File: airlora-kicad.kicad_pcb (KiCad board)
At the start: 4 copper layers, 77 x 77 mm, 125 parts, among them IC1 BALFHB-WL-02D3, J1 12V, J10 I2C, J11 UART2, J2 Conn_Coaxial, J3 Led, J4 SHT, J5 I2C, J6 A_NO2, J7 UART1, J8 A_CO, J9 I2C, Q10 S8050, Q2 S8050, Q3 S8050, Q4 S8050, Q5 S8050, Q6 S8050, Q7 S8050, Q8 S8050, Q9 S8050, SW1 SW_Push, SW2 SW_Slide_DPDT, SW3 SW_Push, U1 TPS7A2633DRVR, U2 TPS54202DDC, U3 TPS7A2633DRVR, U4 BGS12WN6E6327, U6 STM32F103C8Tx, U7 STM32WLE5CCUx, X1 32MHZ, Y1 32.768kHz, Y2 8Mhz

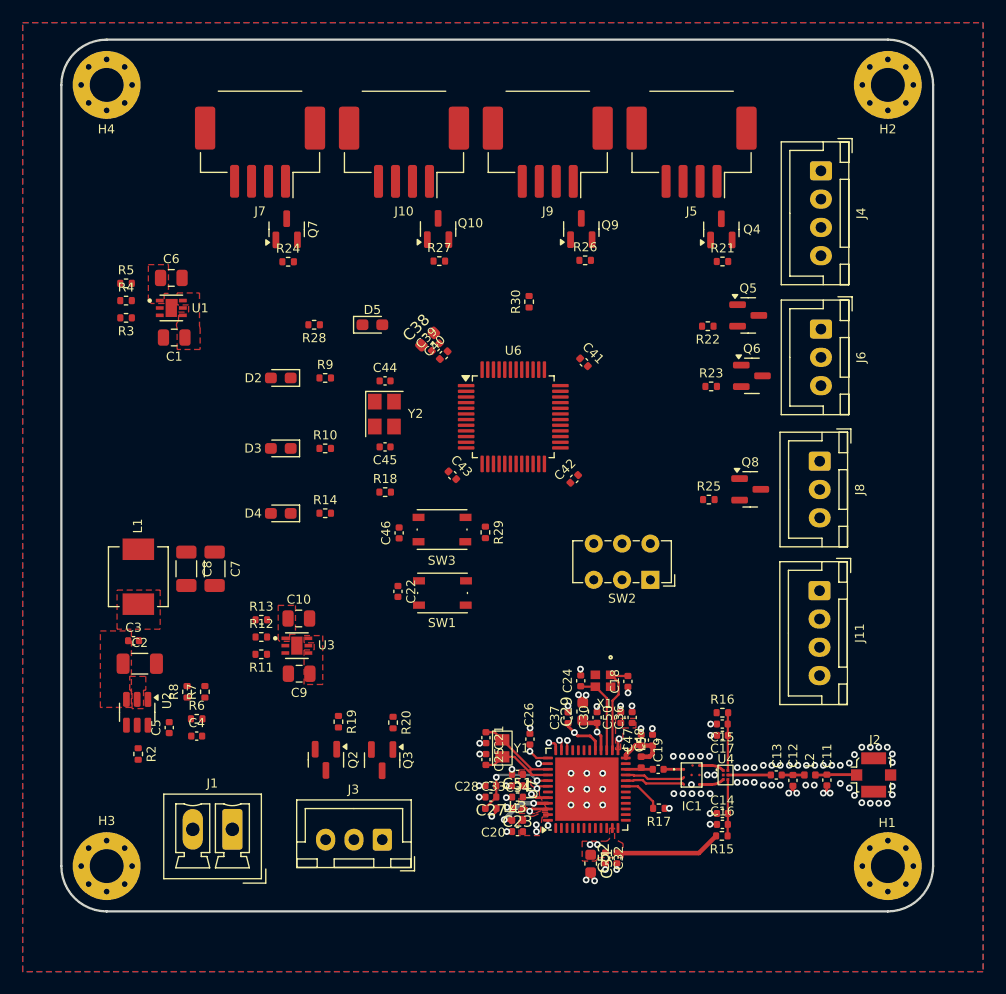
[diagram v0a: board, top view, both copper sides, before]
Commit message: Update PCB layout
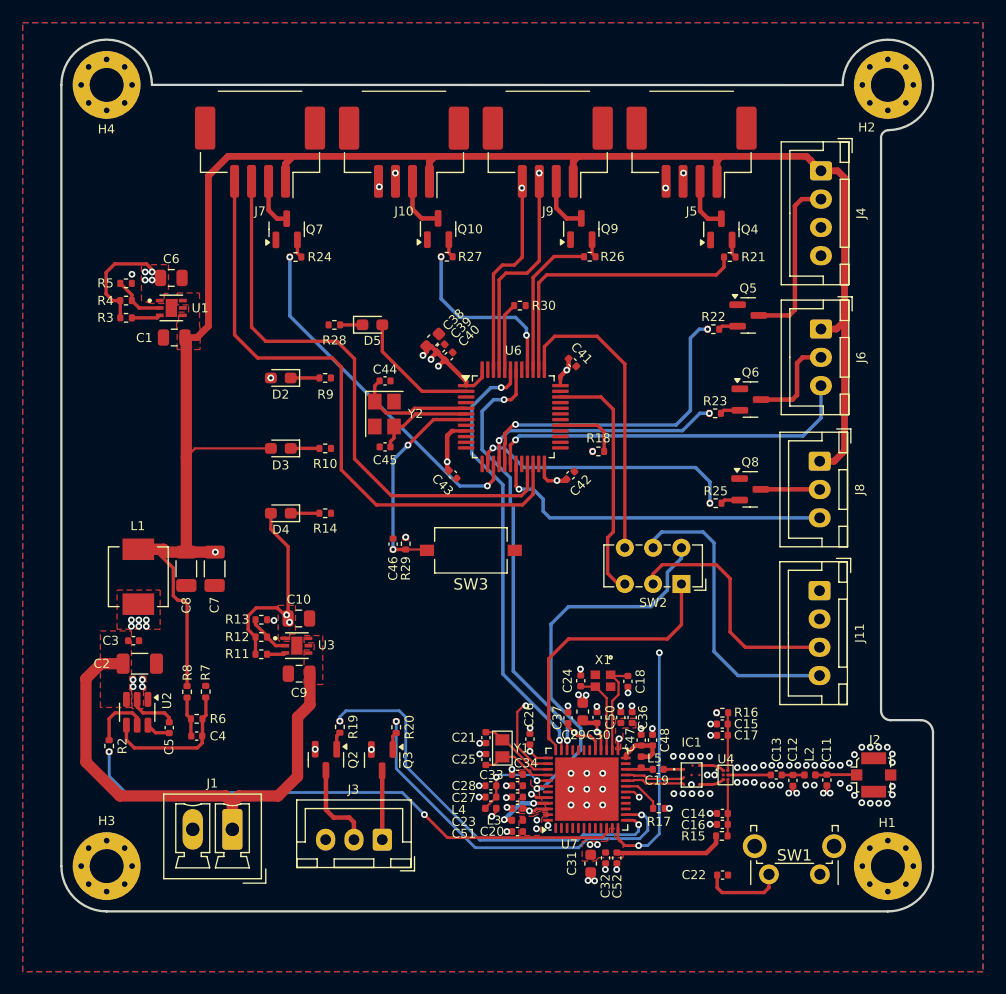
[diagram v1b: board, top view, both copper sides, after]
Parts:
- SW1: footprint Button_Switch_SMD:SW_Push_1P1T_NO_Vertical_Wuerth_434133025816 -> Button_Switch_THT:SW_Tactile_SPST_Angled_PTS645Vx39-2LFS
- SW3: footprint Button_Switch_SMD:SW_Push_1P1T_NO_Vertical_Wuerth_434133025816 -> Button_Switch_SMD:SW_Tactile_SPST_NO_Straight_CK_PTS636Sx25SMTRLFS
- moved SW1 41.6 mm to (127.5, 121.5), turned to 180 degrees
- moved C22 38.1 mm to (118.9, 121.6), turned to 180 degrees
- moved R18 19.2 mm to (108.0, 84.2)
- moved R29 7.11 mm to (90.9, 92.3)
- moved SW3 3.14 mm to (96.7, 92.9), turned to 180 degrees
- moved SW2 2.77 mm to (115.3, 95.9)
- moved R2 2.66 mm to (64.8, 110.2)
- moved R23 2.40 mm to (118.3, 80.8)
- moved Q6 2.10 mm to (121.4, 79.6)
- moved R28 1.79 mm to (84.6, 73.0)
- moved C46 1.12 mm to (89.8, 92.3)
- moved C41 1.02 mm to (105.7, 76.3)
- moved R30 0.88 mm to (101.0, 71.3), turned to 0 degrees
- moved R24 0.78 mm to (81.2, 67.0)
- moved R27 0.77 mm to (94.6, 67.0)
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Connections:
- C18 pad 2: Net-(U7-OSC_OUT) -> Net-(U7-OSC_IN)
- C24 pad 1: Net-(U7-OSC_IN) -> Net-(U7-OSC_OUT)
- J7 pad 3: /AirLora V3/MCU Sub/RX3 -> /AirLora V3/MCU Sub/TX3
- J7 pad 4: /AirLora V3/MCU Sub/TX3 -> /AirLora V3/MCU Sub/RX3
- X1 pad 1: Net-(U7-OSC_OUT) -> Net-(U7-OSC_IN)
- X1 pad 3: Net-(U7-OSC_IN) -> Net-(U7-OSC_OUT)
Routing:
- net +5V: track 0.00 -> 191.1 mm, vias 0 -> 3
- net +3.3V: track 20.7 -> 104.0 mm, vias 7 -> 9
- net +3.3V_HP: track 0.00 -> 73.2 mm, vias 0 -> 12
- net /AirLora V3/MCU Sub/SDA1: track 0.00 -> 61.7 mm, vias 0 -> 3
- net /AirLora V3/MCU Sub/SCL1: track 0.00 -> 61.0 mm, vias 0 -> 3
- net /AirLora V3/MCU Sub/RX3: track 0.00 -> 54.6 mm
- net /AirLora V3/MCU Sub/TX3: track 0.00 -> 51.1 mm
- net /AirLora V3/MCU/PA3: track 0.00 -> 49.0 mm, vias 0 -> 2
- net +12V: track 0.00 -> 44.2 mm
- net Net-(U7-PA4): track 0.00 -> 44.0 mm, vias 0 -> 3
- net /AirLora V3/MCU Sub/SDA2: track 0.95 -> 39.1 mm, vias 1 -> 2
- net /AirLora V3/MCU Sub/SCL2: track 0.88 -> 38.9 mm, vias 1 -> 2
- net /AirLora V3/MCU/PA5: track 0.00 -> 36.4 mm, vias 0 -> 2
- net /AirLora V3/MCU/T_SWCLK: track 1.06 -> 34.3 mm
- net /AirLora V3/MCU/PA6: track 0.00 -> 33.0 mm, vias 0 -> 2
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- added copper zone on In2.Cu, net +3.3V_HP
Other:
- outline, holes or cut-outs redrawn
